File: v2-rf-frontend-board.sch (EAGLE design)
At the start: 155 parts, among them J1 USB_MICROB, J3 ROCKETNET-CONNECTOR-16M, Q1 NTR4101P, T1 ALT4532, T2 ALT4532, U1 MAX2769, U2 SAW, U3 LAN8710A-EZC, U4 7Q-16.368MBG-T, U5 XC2401, U7 LT4619_REDUCED, U8 STM32F4V, U9 LM3480IM3, X1 25 MHz, X2 BU-SMA-H

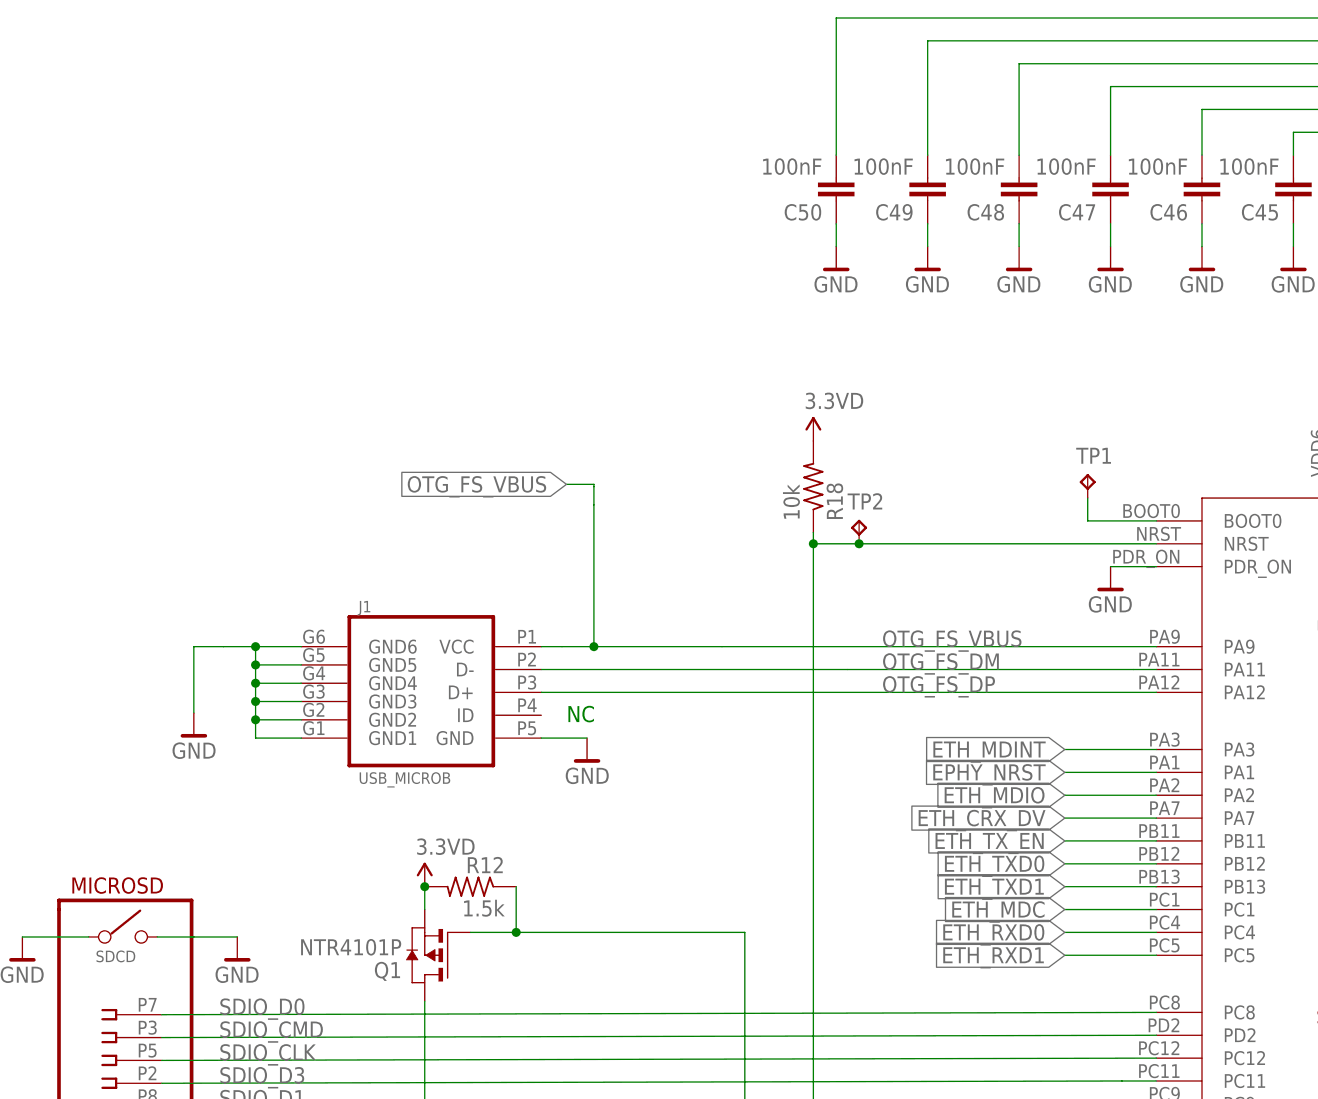
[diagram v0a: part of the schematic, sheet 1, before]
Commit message: Updated microUSB symbol and library. Package not finalized.
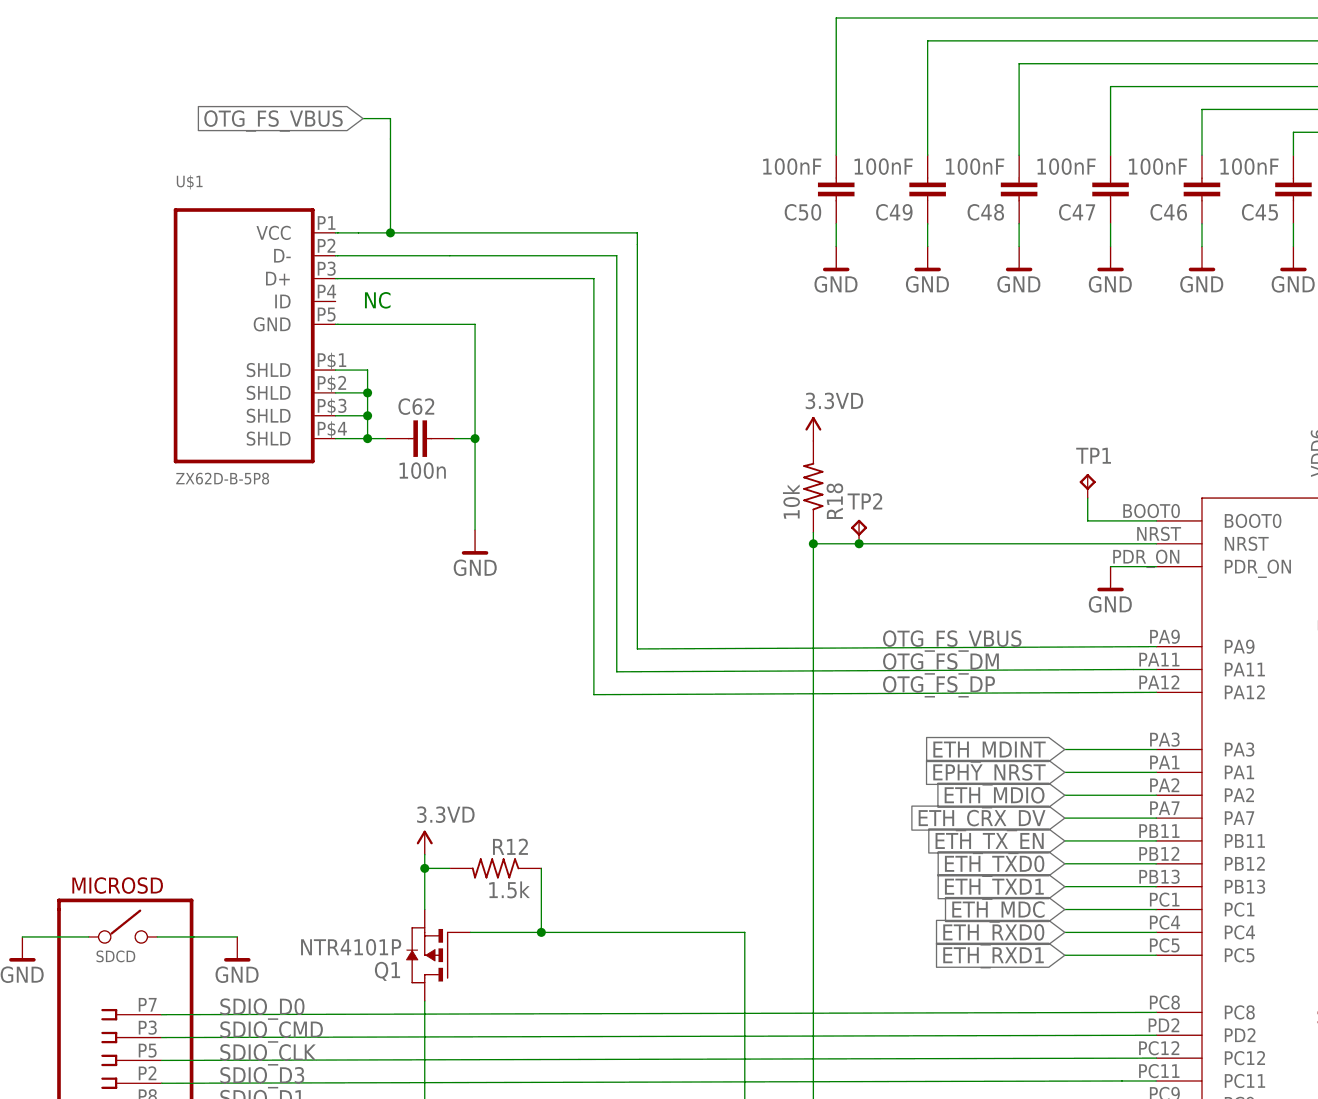
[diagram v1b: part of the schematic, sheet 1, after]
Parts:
- removed J1: USB_MICROB, con-hirose-microusb:ZX62D-B-5P8
- added C62: 100n, rcl:C-EUC0402
- added U$1: ZX62D-B-5P8, con-hirose-microusb:ZX62D-B-5P8
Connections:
- new net SHLD: C62.2, U$1.SHLD@1, U$1.SHLD@2, U$1.SHLD@3, U$1.SHLD@4
- net GND: now also C62.1, U$1.GND; no longer J1.GND, J1.GND1, J1.GND2, J1.GND3, J1.GND4, J1.GND5, J1.GND6
- net OTG_FS_DM: now also U$1.D-; no longer J1.D-
- net OTG_FS_DP: now also U$1.D+; no longer J1.D+
- net OTG_FS_VBUS: now also U$1.VCC; no longer J1.VCC
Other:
- moved on the sheet: R12
